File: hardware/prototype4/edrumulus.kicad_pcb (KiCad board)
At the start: 2 copper layers, 65 x 56.5 mm, 67 parts, among them J1 Trigger Connector, J2 Raspberry Pi GPIO pins, U1 ESP32-DEVKIT-V1

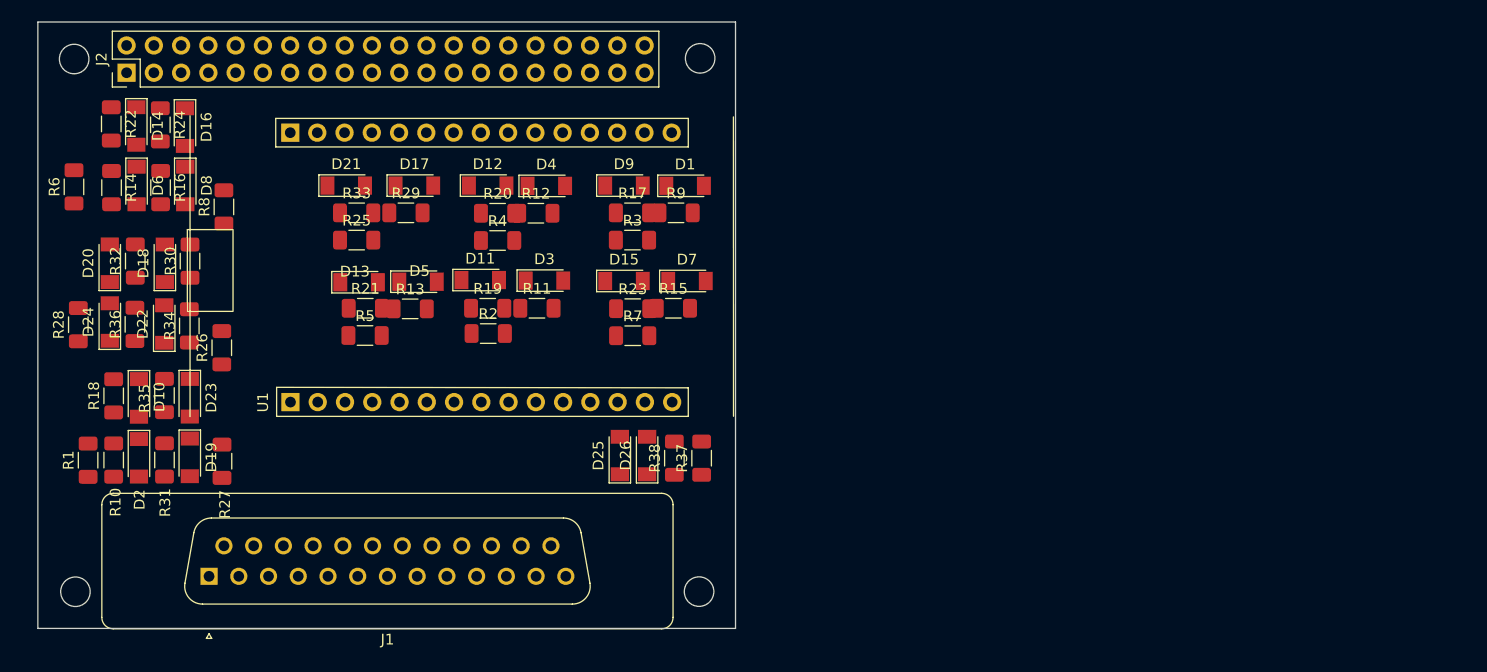
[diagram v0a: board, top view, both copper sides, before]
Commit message: some more routing
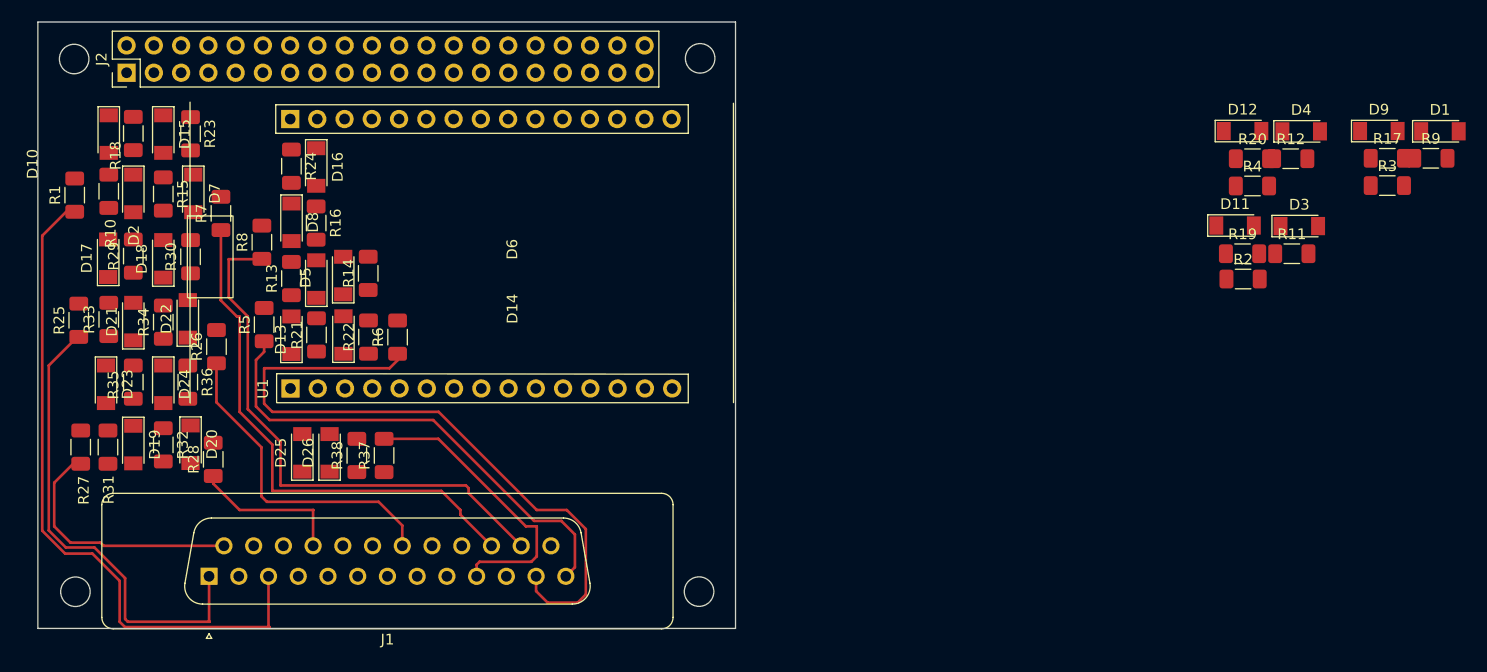
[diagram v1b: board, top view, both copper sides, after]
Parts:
- moved D1 70.5 mm to (237.3, 83.8)
- moved D3 70.5 mm to (224.2, 92.7)
- moved D9 70.5 mm to (231.6, 83.8)
- moved R12 70.5 mm to (223.4, 86.4)
- moved R20 70.5 mm to (219.8, 86.4)
- moved R4 70.5 mm to (219.8, 88.9)
- moved R9 70.5 mm to (236.5, 86.4)
- moved D11 70.5 mm to (218.2, 92.6)
- moved D12 70.5 mm to (218.9, 83.8)
- moved D4 70.5 mm to (224.4, 83.8)
- moved R11 70.5 mm to (223.5, 95.2)
- moved R17 70.5 mm to (232.4, 86.4)
- moved R19 70.5 mm to (218.9, 95.2)
- moved R2 70.5 mm to (219.0, 97.6)
- moved R3 70.5 mm to (232.4, 88.9)
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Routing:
- net CRASH1-TIP: track 0.00 -> 64.3 mm
- net SNARE-TIP: track 0.00 -> 63.3 mm
- net RIDE-TIP: track 0.00 -> 51.2 mm
- net RIDE-RING: track 0.00 -> 49.6 mm
- net CRASH1-RING: track 0.00 -> 45.3 mm
- net KICK-TIP: track 0.00 -> 44.3 mm
- net TOM3-TIP: track 0.00 -> 30.3 mm
- net HI-HAT-CONTROL-TIP: track 0.00 -> 27.4 mm
- net TOM1-TIP: track 0.00 -> 23.8 mm
- net TOM2-TIP: track 0.00 -> 14.4 mm
